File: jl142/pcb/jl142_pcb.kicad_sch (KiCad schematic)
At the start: 86 parts, among them SW12 SWITCH_PUSH, SW13 SWITCH_PUSH, SW14 SWITCH_PUSH, SW17 SWITCH_PUSH, SW18 SWITCH_PUSH, SW19 SWITCH_PUSH, SW2 SWITCH_PUSH, SW20 SWITCH_PUSH, SW22 SWITCH_PUSH, SW23 SWITCH_PUSH, SW24 SWITCH_PUSH, SW25 SWITCH_PUSH, SW27 SWITCH_PUSH, SW28 SWITCH_PUSH, SW29 SWITCH_PUSH, SW3 SWITCH_PUSH, SW30 SWITCH_PUSH, SW34 SWITCH_PUSH, SW35 SWITCH_PUSH, SW36 SWITCH_PUSH, SW37 SWITCH_PUSH, SW39 SWITCH_PUSH, SW4 SWITCH_PUSH, SW40 SWITCH_PUSH, SW41 SWITCH_PUSH, SW42 SWITCH_PUSH, SW44 SWITCH_PUSH, SW45 SWITCH_PUSH, SW46 SWITCH_PUSH, SW47 SWITCH_PUSH, SW49 SWITCH_PUSH, SW50 SWITCH_PUSH, SW51 SWITCH_PUSH, SW54 SWITCH_PUSH, SW55 SWITCH_PUSH, SW56 SWITCH_PUSH, SW59 SWITCH_PUSH, SW60 SWITCH_PUSH, SW61 SWITCH_PUSH, SW7 SWITCH_PUSH, SW8 SWITCH_PUSH, SW9 SWITCH_PUSH, U1 ARDUINO_PRO_MICRO

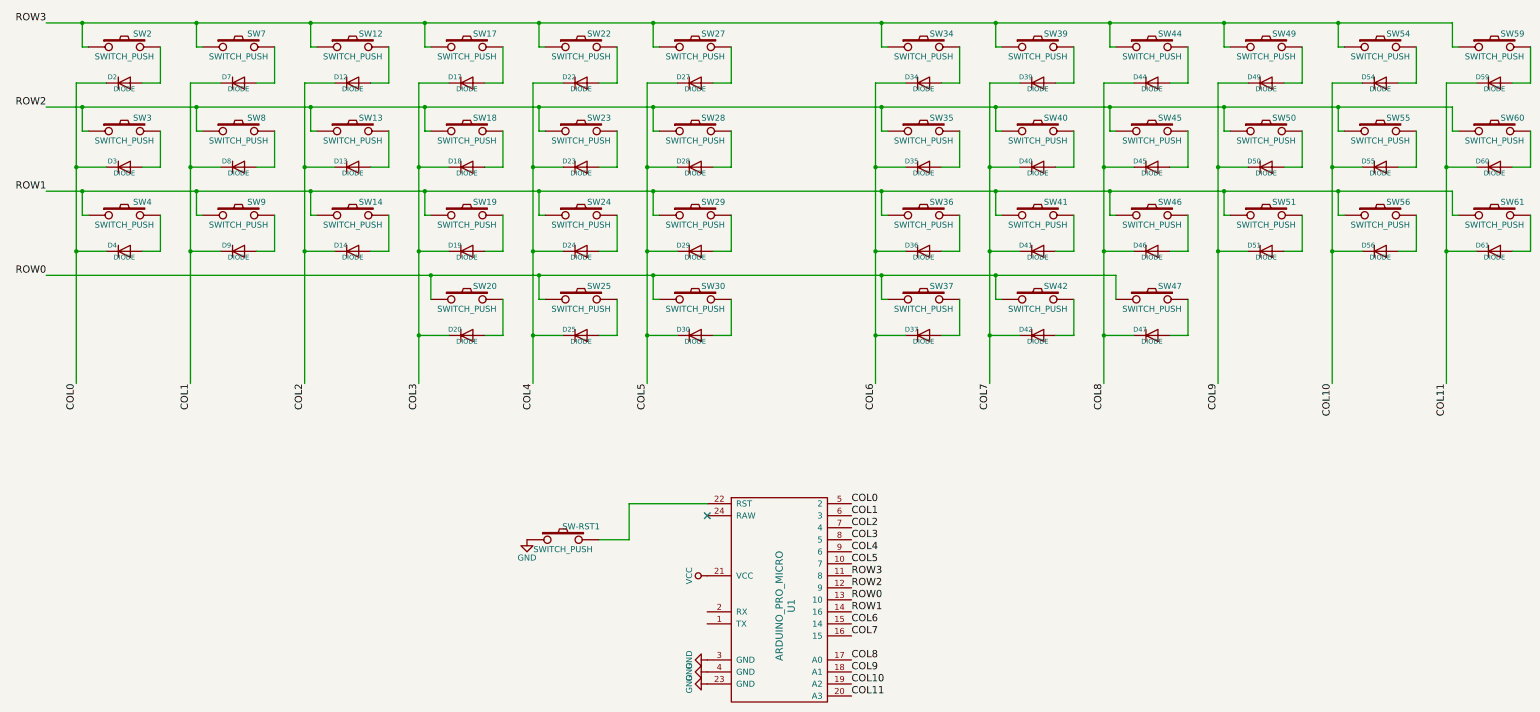
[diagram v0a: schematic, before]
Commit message: Moved files around.
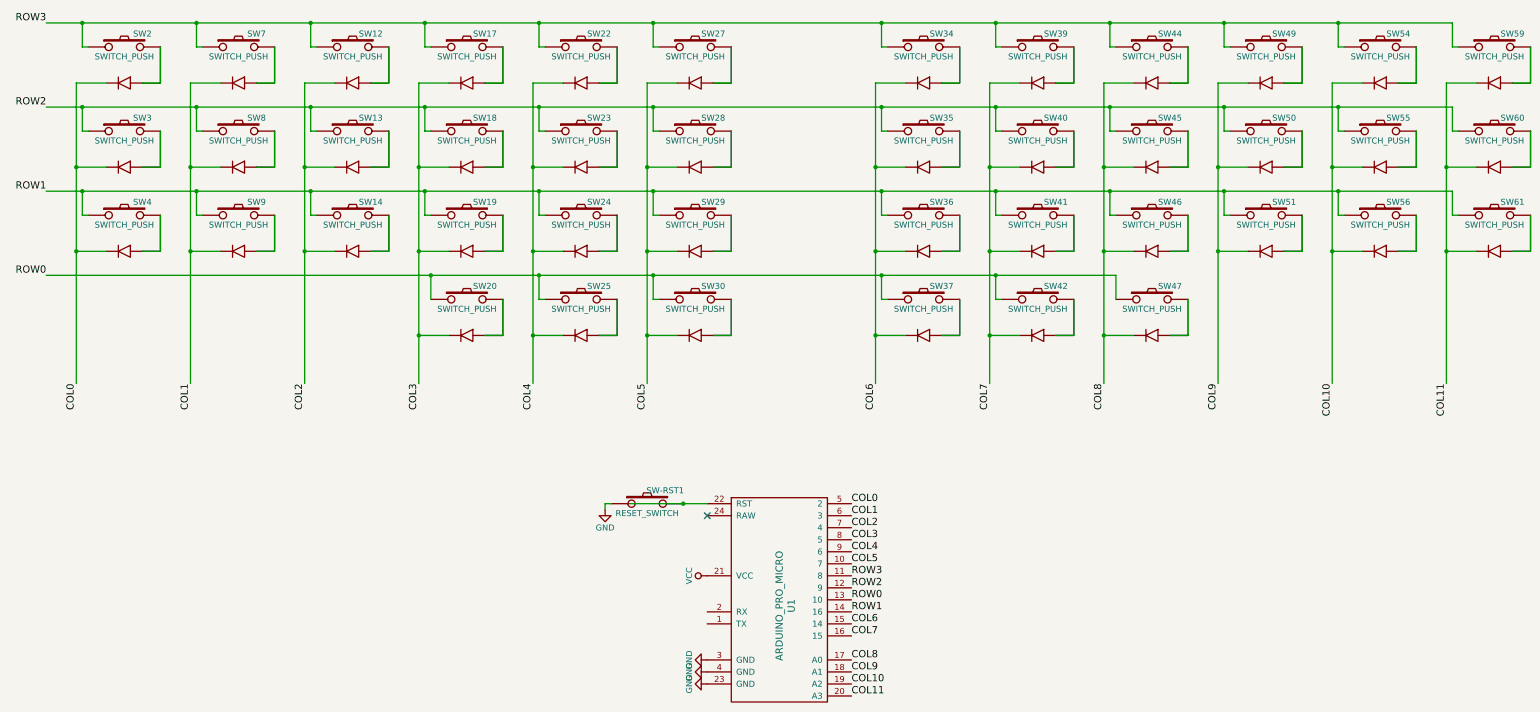
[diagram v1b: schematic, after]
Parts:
- removed D12, D13, D14, D17, D18, D19, D2, D20, D22, D23, D24, D25, D27, D28, D29, D3, D30, D34, D35, D36, D37, D39, D4, D40, D41, D42, D44, D45, D46, D47, D49, D50, D51, D54, D55, D56, D59, D60, D61, D7, D8, D9: DIODE, Diode_THT:D_DO-35_SOD27_P7.62mm_Horizontal, symbol Diode:1N4148
- SW-RST1: value SWITCH_PUSH -> RESET_SWITCH
- SW12, SW13, SW14, SW17, SW18, SW19, SW2, SW20, SW22, SW23, SW24, SW25, SW27, SW28, SW29, SW3, SW30, SW34, SW35, SW36, SW37, SW39, SW4, SW40, SW41, SW42, SW44, SW45, SW46, SW47, SW49, SW50, SW51, SW54, SW55, SW56, SW59, SW60, SW61, SW7, SW8, SW9: footprint footprints:Kailh_socket_PG1350_optional -> footprints:kailh_choc_with_diode; symbol symbols:SWITCH_PUSH -> symbols:SWITCH_WITH_DIODE
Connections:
- net COL0: now also SW2.3 (K), SW3.3 (K), SW4.3 (K)
- net COL1: now also SW7.3 (K), SW8.3 (K), SW9.3 (K)
- net COL10: now also SW54.3 (K), SW55.3 (K), SW56.3 (K)
- net COL11: now also SW59.3 (K), SW60.3 (K), SW61.3 (K)
- net COL2: now also SW12.3 (K), SW13.3 (K), SW14.3 (K)
- net COL3: now also SW17.3 (K), SW18.3 (K), SW19.3 (K), SW20.3 (K)
- net COL4: now also SW22.3 (K), SW23.3 (K), SW24.3 (K), SW25.3 (K)
- net COL5: now also SW27.3 (K), SW28.3 (K), SW29.3 (K), SW30.3 (K)
- net COL6: now also SW34.3 (K), SW35.3 (K), SW36.3 (K), SW37.3 (K)
- net COL7: now also SW39.3 (K), SW40.3 (K), SW41.3 (K), SW42.3 (K)
- net COL8: now also SW44.3 (K), SW45.3 (K), SW46.3 (K), SW47.3 (K)
- net COL9: now also SW49.3 (K), SW50.3 (K), SW51.3 (K)
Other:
- moved on the sheet: SW-RST1
